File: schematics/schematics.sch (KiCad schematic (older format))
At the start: 6 parts

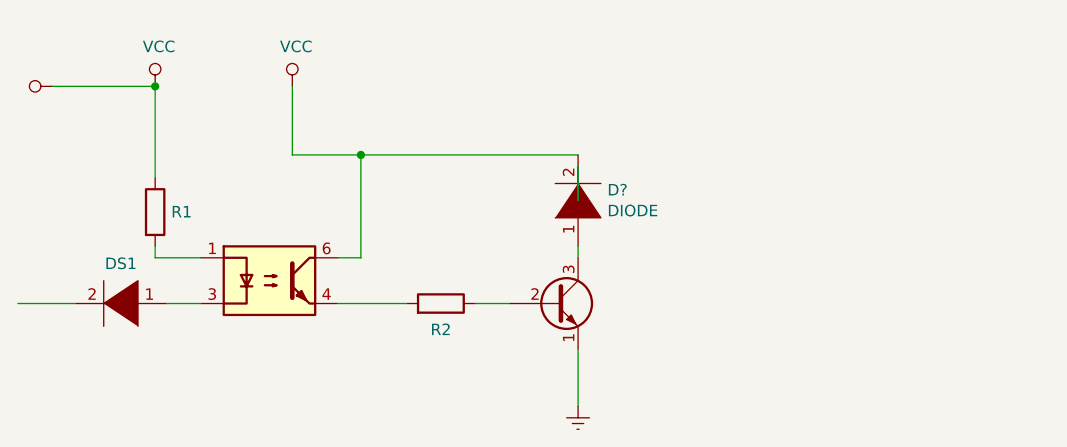
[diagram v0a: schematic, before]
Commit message: Final wersion of the pump circuit
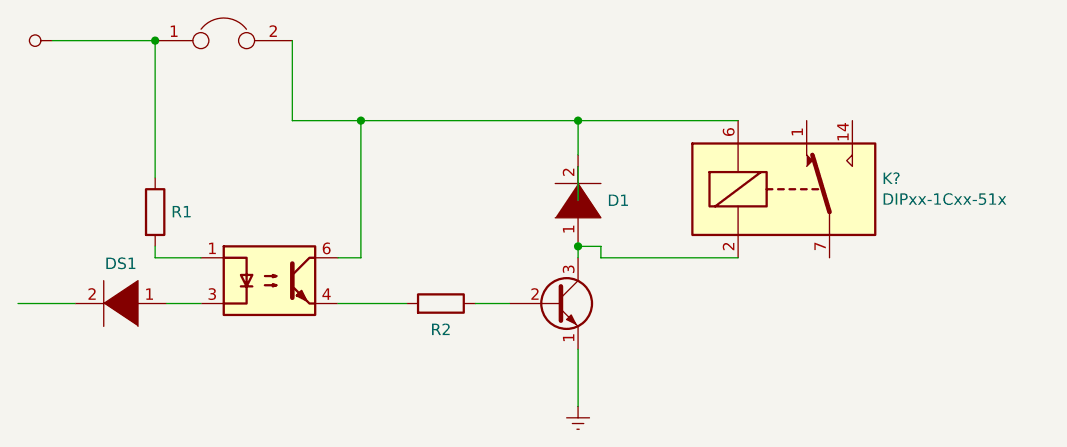
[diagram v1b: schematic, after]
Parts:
- added JP?: Jumper, symbol Device:Jumper
- added K?: DIPxx-1Cxx-51x, Relay_THT:Relay_StandexMeder_DIP_LowProfile, symbol Relay:DIPxx-1Cxx-51x
- gave numbers to parts that had none: 1
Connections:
- wire segments 16 -> 21
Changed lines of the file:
@@
-	1    0    0    -1
-$EndComp
-$Comp
-L power:VCC #PWR?
-U 1 1 5C8BCB84
-P 4700 3750
-F 0 "#PWR?" H 4700 3600 50  0001 C CNN
-F 1 "VCC" H 4717 3923 50  0000 C CNN
-F 2 "" H 4700 3750 50  0001 C CNN
-F 3 "" H 4700 3750 50  0001 C CNN
-	1    4700 3750
 	1    0    0    -1
 $EndComp
 Wire Wire Line
-	4700 3750 4250 3750
-Connection ~ 4700 3750
+	4700 3550 4250 3550
 $Comp
 L power:VCC #PWR?
 U 1 1 5C8BE04C
-P 4250 3750
-F 0 "#PWR?" H 4250 3600 50  0001 C CNN
-F 1 "VCC" V 4268 3877 50  0001 L CNN
-F 2 "" H 4250 3750 50  0001 C CNN
-F 3 "" H 4250 3750 50  0001 C CNN
-	1    4250 3750
+P 4250 3550
+F 0 "#PWR?" H 4250 3400 50  0001 C CNN
+F 1 "VCC" V 4268 3677 50  0001 L CNN
+F 2 "" H 4250 3550 50  0001 C CNN
+F 3 "" H 4250 3550 50  0001 C CNN
+	1    4250 3550
 	0    -1   -1   0
 $EndComp
@@
 	5500 4500 5600 4500
 Wire Wire Line
-	5600 4050 5300 4050
-$Comp
-L power:VCC #PWR?
-U 1 1 5C8C0019
-P 5300 3750
-F 0 "#PWR?" H 5300 3600 50  0001 C CNN
-F 1 "VCC" H 5317 3923 50  0000 C CNN
-F 2 "" H 5300 3750 50  0001 C CNN
-F 3 "" H 5300 3750 50  0001 C CNN
-	1    5300 3750
-	1    0    0    -1
-$EndComp
-Wire Wire Line
-	5600 4050 6550 4050
-Connection ~ 5600 4050
-Wire Wire Line
 	6550 4500 6550 4450
 $Comp
-L pspice:DIODE D?
+L pspice:DIODE D1
 U 1 1 5C8C3A6E
 P 6550 4250
-F 0 "D?" V 6596 4122 50  0000 R CNN
-F 1 "DIODE" V 6505 4122 50  0000 R CNN
+F 0 "D1" V 6550 4122 50  0000 R CNN
+F 1 "DIODE" V 6505 4122 50  0001 R CNN
 F 2 "" H 6550 4250 50  0001 C CNN
 F 3 "~" H 6550 4250 50  0001 C CNN
@@
 $EndComp
 Wire Wire Line
-	5300 3750 5300 4050
+	6550 4100 6550 4250
+$Comp
+L Device:Jumper JP?
+U 1 1 5C8CFC95
+P 5000 3550
+F 0 "JP?" H 5000 3814 50  0001 C CNN
+F 1 "Jumper" H 5000 3723 50  0001 C CNN
+F 2 "" H 5000 3550 50  0001 C CNN
+F 3 "~" H 5000 3550 50  0001 C CNN
+	1    5000 3550
+	1    0    0    -1
+$EndComp
+$Comp
+L Relay:DIPxx-1Cxx-51x K?
+U 1 1 5C8D3DB8
+P 7450 4200
+F 0 "K?" H 7880 4246 50  0000 L CNN
+F 1 "DIPxx-1Cxx-51x" H 7880 4155 50  0000 L CNN
+F 2 "Relay_THT:Relay_StandexMeder_DIP_LowProfile" H 7900 4150 50  0001 L CNN
+F 3 "https://standexelectronics.com/wp-content/uploads/datasheet_reed_relay_DIP.pdf" H 7450 4200 50  0001 C CNN
+	1    7450 4200
+	1    0    0    -1
+$EndComp
 Wire Wire Line
-	4700 3750 4700 4150
+	5300 3900 5600 3900
 Wire Wire Line
-	5600 4050 5600 4500
+	5300 3550 5300 3900
 Wire Wire Line
-	6550 4100 6550 4250
+	6550 4050 6550 3900
+Wire Wire Line
+	4700 3550 4700 4150
+Connection ~ 4700 3550
+Wire Wire Line
+	5600 3900 5600 4500
+Connection ~ 5600 3900
+Wire Wire Line
+	5600 3900 6550 3900
+Wire Wire Line
+	7250 3900 6550 3900
+Connection ~ 6550 3900
+Wire Wire Line
+	7250 4500 6650 4500
+Wire Wire Line
+	6650 4500 6650 4450
+Wire Wire Line
+	6650 4450 6550 4450
+Connection ~ 6550 4450
 $EndSCHEMATC
